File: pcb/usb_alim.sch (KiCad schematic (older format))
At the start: 0 parts

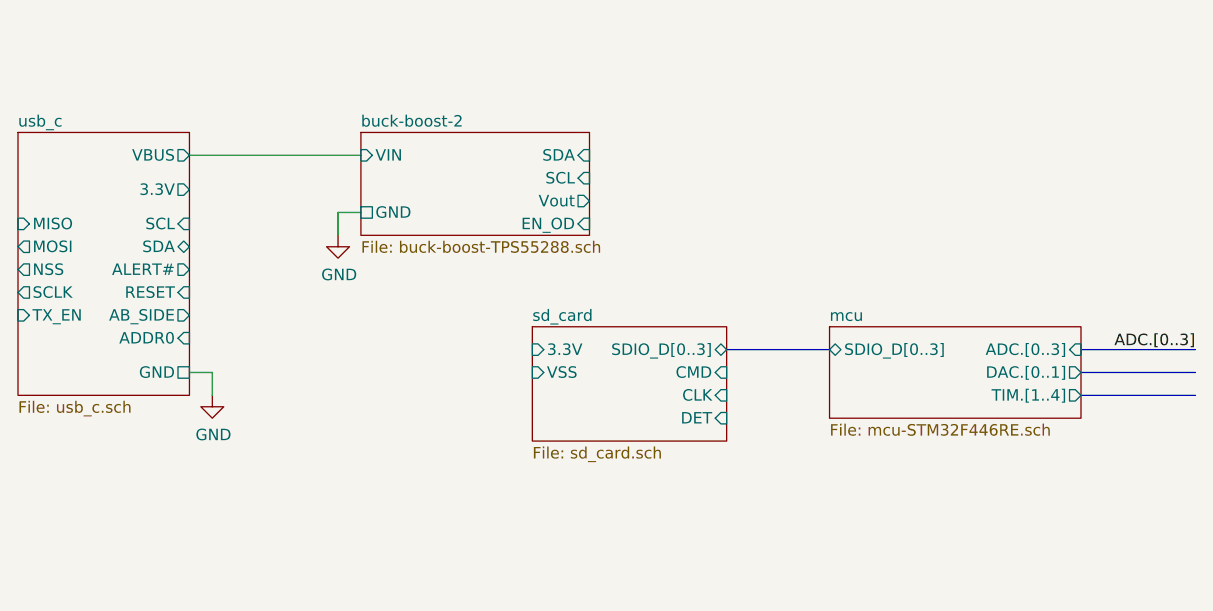
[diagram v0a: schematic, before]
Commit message: [PCB] minor changes
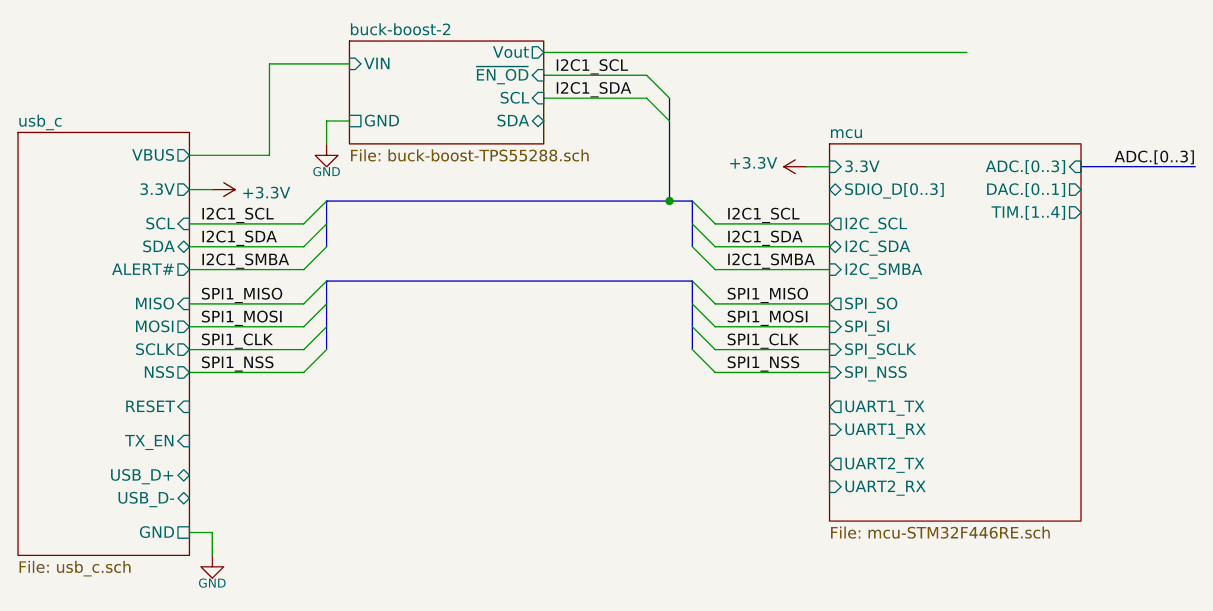
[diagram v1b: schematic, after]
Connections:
- net labels added: +3.3V, I2C1_SCL, I2C1_SDA, I2C1_SMBA, SPI1_CLK, SPI1_MISO, SPI1_MOSI, SPI1_NSS
- wire segments 5 -> 26
